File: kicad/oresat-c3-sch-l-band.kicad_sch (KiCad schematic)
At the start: 87 parts, among them U15 Qorvo 856930, U16 AX5043, U17 SI4112-GM, U2 BP0805A1308, U29 TQP3M9036, U3 BP0805A1308, U4 BGB741L7ESD, U5 BP0805A1308, U7 MAC-24+

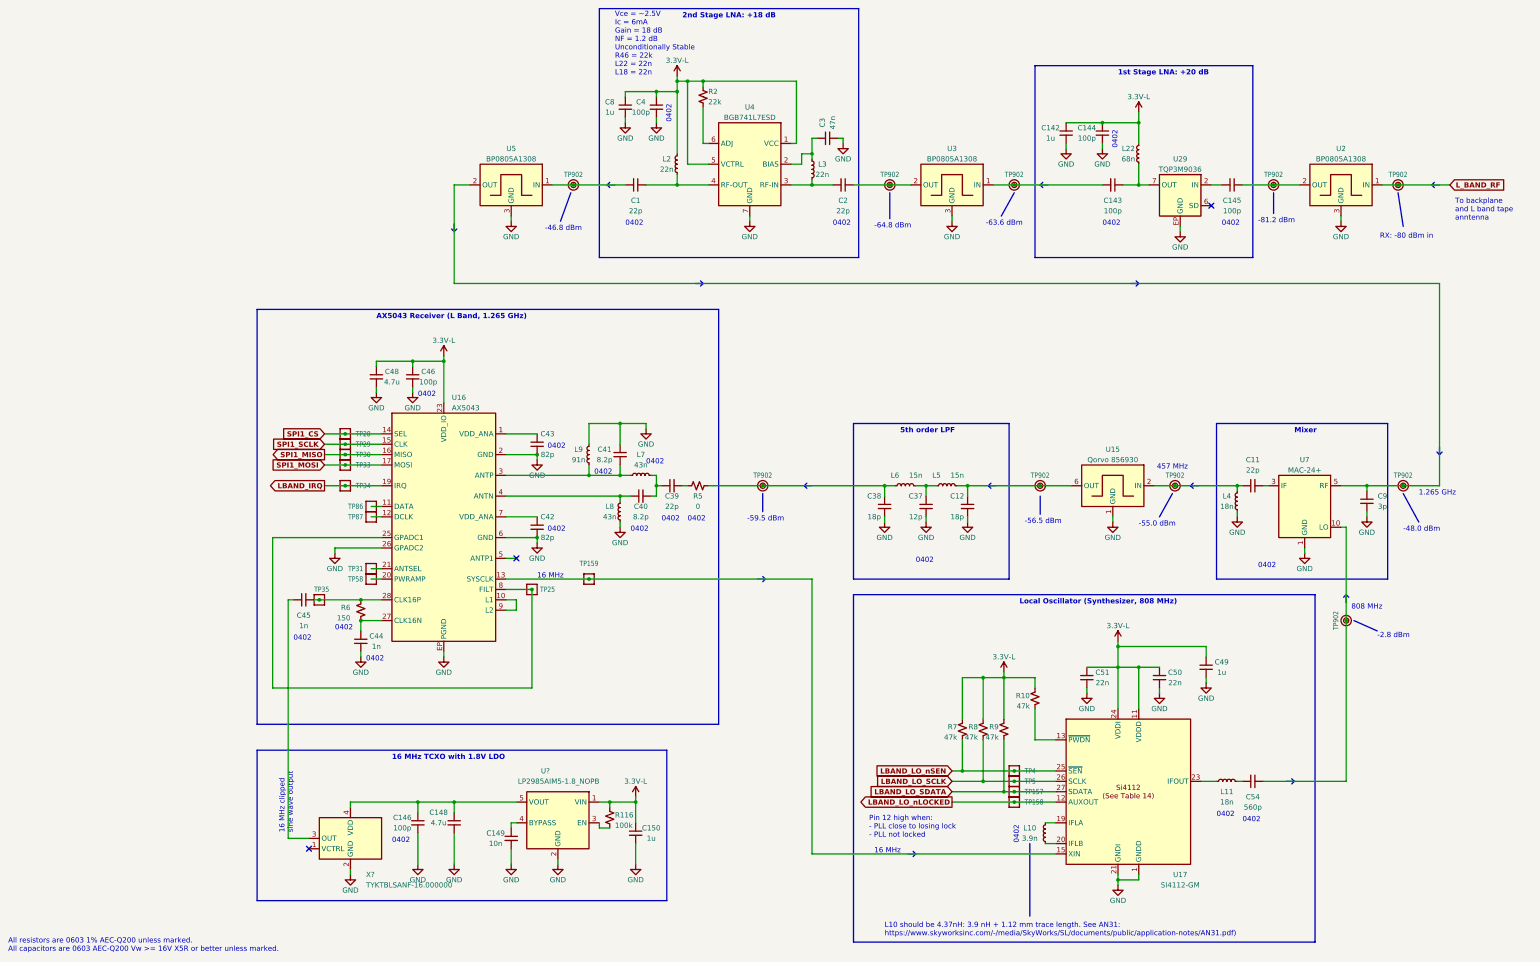
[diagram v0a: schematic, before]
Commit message: Added Oresat symbol lib. Removed any L-band related components from pcb and schematic
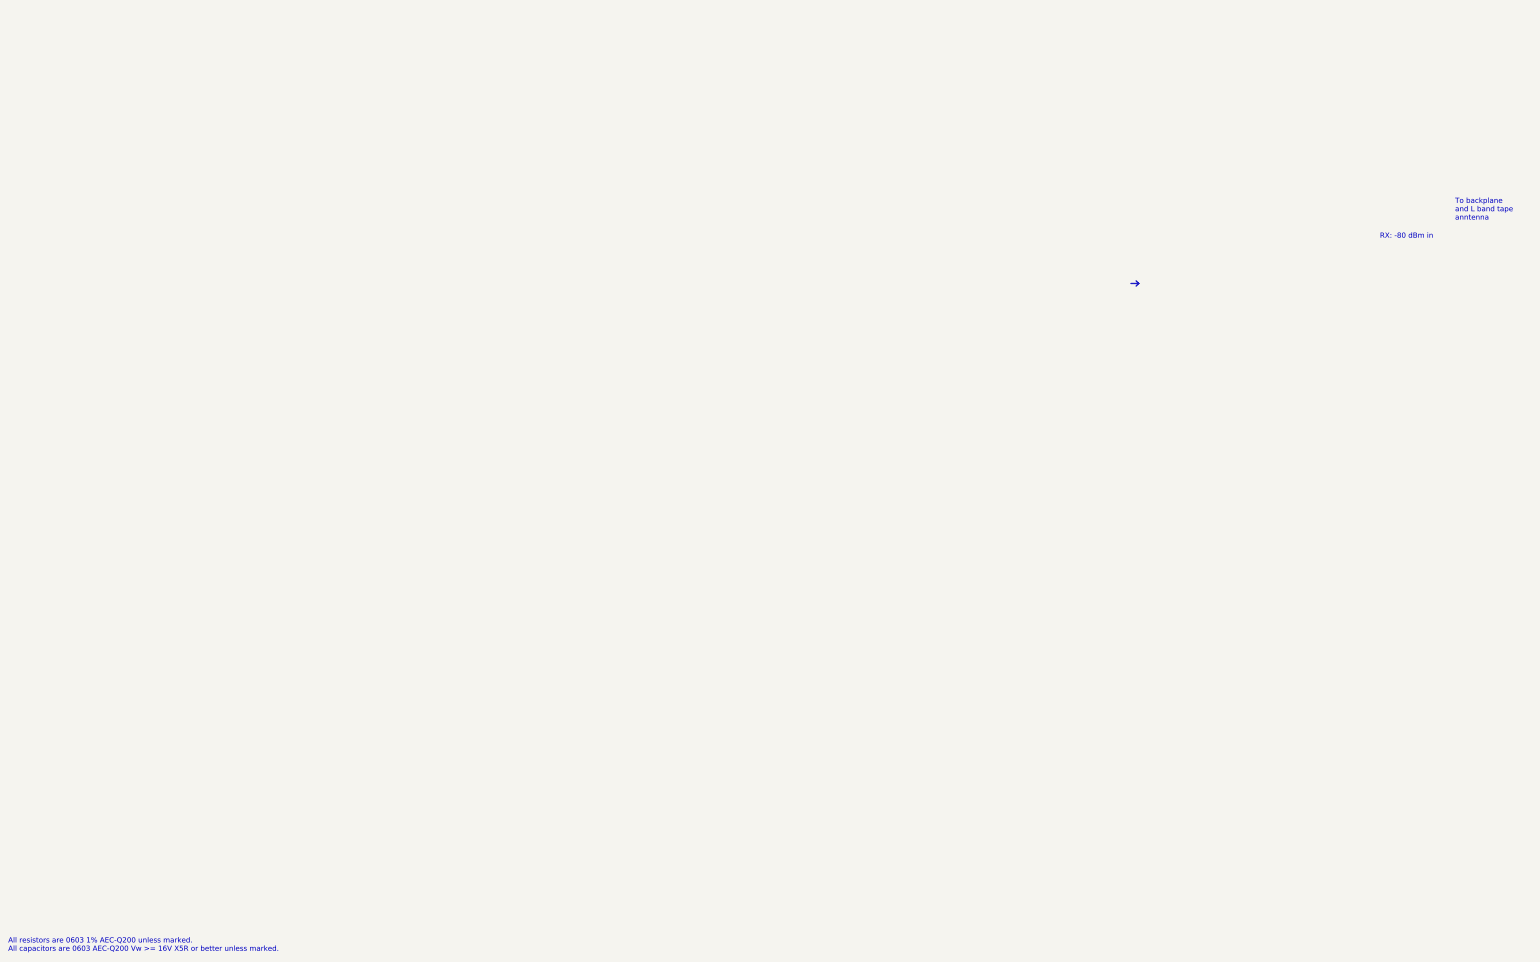
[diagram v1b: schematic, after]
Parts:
- removed C1, C11, C2, C39: 22p, Capacitor_SMD:C_0402_1005Metric, symbol Device:C_Small
- removed C12, C38: 18p, Capacitor_SMD:C_0402_1005Metric, symbol Device:C_Small
- removed C142, C150, C49, C8: 1u, Capacitor_SMD:C_0603_1608Metric, symbol Device:C_Small
- removed C143, C144, C145, C146, C4, C46: 100p, Capacitor_SMD:C_0402_1005Metric, symbol Device:C_Small
- removed C148, C48: 4.7u, Capacitor_SMD:C_0603_1608Metric, symbol Device:C_Small
- removed C149: 10n, Capacitor_SMD:C_0603_1608Metric, symbol Device:C_Small
- removed C3: 47n, Capacitor_SMD:C_0603_1608Metric, symbol Device:C_Small
- removed C37: 12p, Capacitor_SMD:C_0402_1005Metric, symbol Device:C_Small
- removed C40, C41: 8.2p, Capacitor_SMD:C_0402_1005Metric, symbol Device:C_Small
- removed C42, C43: 82p, Capacitor_SMD:C_0402_1005Metric, symbol Device:C_Small
- removed C44, C45: 1n, Capacitor_SMD:C_0402_1005Metric, symbol Device:C_Small
- removed C50, C51: 22n, Capacitor_SMD:C_0603_1608Metric, symbol Device:C_Small
- removed C54: 560p, Capacitor_SMD:C_0402_1005Metric, symbol Device:C_Small
- removed C9: 3p, Capacitor_SMD:C_0402_1005Metric, symbol Device:C_Small
- removed L10: 3.9n, Inductor_SMD:L_0402_1005Metric, symbol Device:L_Small
- removed L11, L4: 18n, Inductor_SMD:L_0402_1005Metric, symbol Device:L_Small
- removed L2, L3: 22n, Inductor_SMD:L_0603_1608Metric, symbol Device:L_Small
- removed L22: 68n, Inductor_SMD:L_0603_1608Metric, symbol Device:L_Small
- removed L5, L6: 15n, Inductor_SMD:L_0402_1005Metric, symbol Device:L_Small
- removed L7: 43n, Inductor_SMD:L_0402_1005Metric, symbol Device:L_Small
- removed L8: 43n, Inductor_SMD:L_0603_1608Metric, symbol Device:L_Small
- removed L9: 91n, Inductor_SMD:L_0603_1608Metric, symbol Device:L_Small
- removed R10, R7, R8, R9: 47k, Resistor_SMD:R_0603_1608Metric, symbol Device:R_Small_US
- removed R116: 100k, Resistor_SMD:R_0603_1608Metric, symbol Device:R_Small_US
- removed R2: 22k, Resistor_SMD:R_0603_1608Metric, symbol Device:R_Small_US
- removed R5: 0, Resistor_SMD:R_0402_1005Metric, symbol Device:R_Small_US
- removed R6: 150, Resistor_SMD:R_0402_1005Metric, symbol Device:R_Small_US
- removed TP157, TP158, TP159, TP25, TP28, TP29, TP30, TP31, TP33, TP34, TP35, TP4, TP5, TP58, TP86, TP87: Test-Point, oresat-misc:TestPoint_Pad_D1.0mm, symbol oresat-misc:Test-Point-1mm-round
- removed TP902 (x10): ~, oresat-misc:TestPoint_RF_Probe, symbol oresat-misc:Test-Point-RF-Probe-Stripline
- removed U15: Qorvo 856930, oresat-ics:856930-saw-filter, symbol oresat-passives:856930
- removed U16: AX5043, oresat-ics:U-AX5043-QFN28-5X5-WITH-CENTER-PAD, symbol oresat-ics:AX5043
- removed U17: SI4112-GM, Package_DFN_QFN:QFN-28-1EP_5x5mm_P0.5mm_EP3.35x3.35mm_ThermalVias, symbol oresat-ics:SI4112
- removed U2, U3, U5: BP0805A1308, oresat-ics:BP0805, symbol oresat-passives:BP0805A1308
- removed U29: TQP3M9036, oresat-ics:U-Qorvo-TQP3M9036-QFN-8-MO-220E, symbol oresat-ics:TQP3M9036
- removed U4: BGB741L7ESD, oresat-ics:Infineon-PG-TSLP-7-LNA, symbol oresat-ics:BGB741L7ESD
- removed U7: MAC-24+, oresat-ics:MAC-24+, symbol oresat-ics:MAC-24+
- removed U?: LP2985AIM5-1.8_NOPB, Package_TO_SOT_SMD:SOT-23-5, symbol oresat-ics:LP2985-N
- removed X?: TYKTBLSANF-16.000000, oresat-ics:X_TCXO_SMD_Taitien_2.5x2.0mm, symbol oresat-ics:Taiten-TY-Series-TXCO
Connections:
- no-connect marks 3 -> 0
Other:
- note removed: "-2.8 dBm"
- note removed: "-46.8 dBm"
- note removed: "-48.0 dBm"
- note removed: "-55.0 dBm"
- note removed: "-56.5 dBm"
- note removed: "-59.5 dBm"
- note removed: "-63.6 dBm"
- note removed: "-64.8 dBm"
- note removed: "-81.2 dBm"
- note removed: "0402"
- note removed: "1.265 GHz"
- note removed: "16 MHz"
- note removed: "16 MHz TCXO with 1.8V LDO"
- note removed: "16 MHz clipped sine wave output"
- note removed: "1st Stage LNA: +20 dB"
- note removed: "2nd Stage LNA: +18 dB"
- note removed: "457 MHz"
- note removed: "5th order LPF"
- note removed: "808 MHz"
- note removed: "AX5043 Receiver (L Band, 1.265 GHz)"
- note removed: "L10 should be 4.37nH: 3.9 nH + 1.12 mm trace length. See AN31: https://www.skyworksinc.com/-/media/SkyWorks/SL/documents/public/application-notes/AN31.pdf)"
- note removed: "Local Oscillator (Synthesizer, 808 MHz)"
- note removed: "Mixer"
- note removed: "Pin 12 high when: - PLL close to losing lock - PLL not locked"
- note removed: "Vce = ~2.5V Ic = 6mA Gain = 18 dB NF = 1.2 dB Unconditionally Stable R46 = 22k L22 = 22n L18 = 22n"
